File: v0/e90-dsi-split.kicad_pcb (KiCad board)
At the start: 2 copper layers, 33.9 x 22.1 mm, 12 parts, among them J1 3-2328724-1, J2 BM23PF0.8-40DP-0.35V_51_, J3 I2C Pinstack, J4 GPIO Pinstack

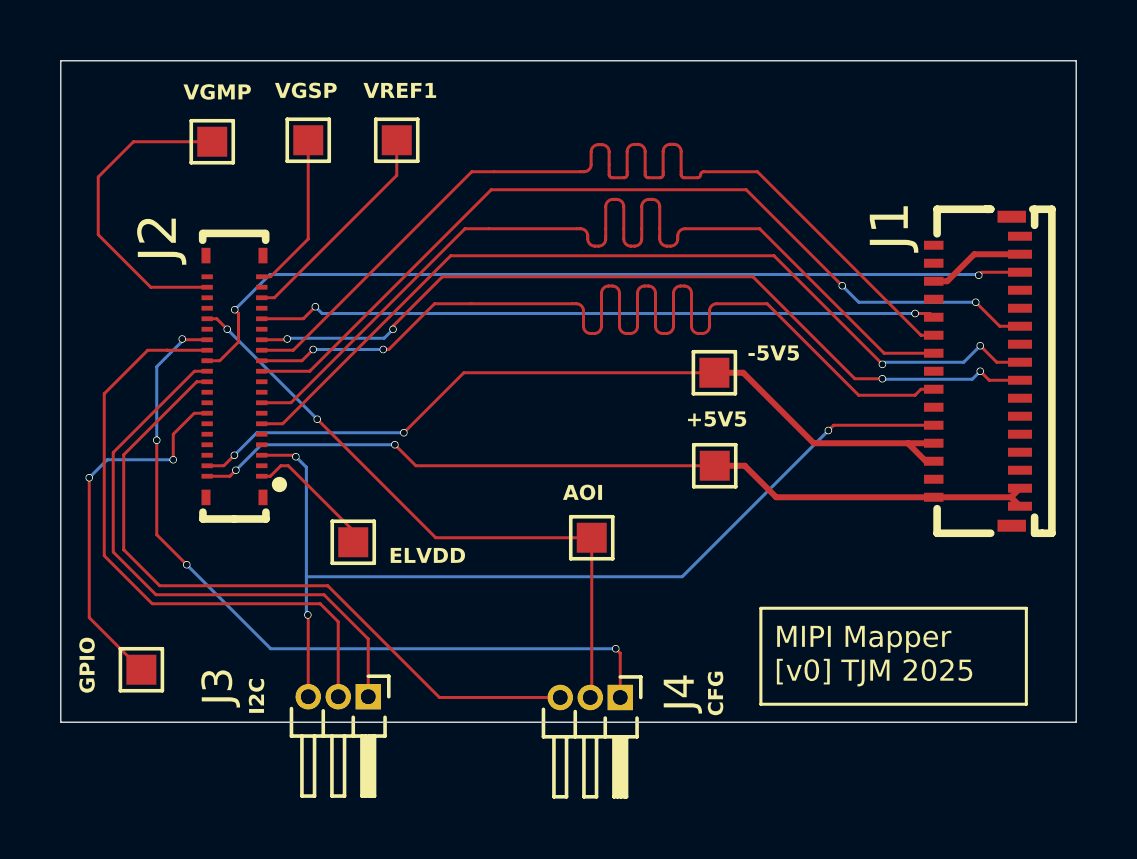
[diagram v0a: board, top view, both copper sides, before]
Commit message: next
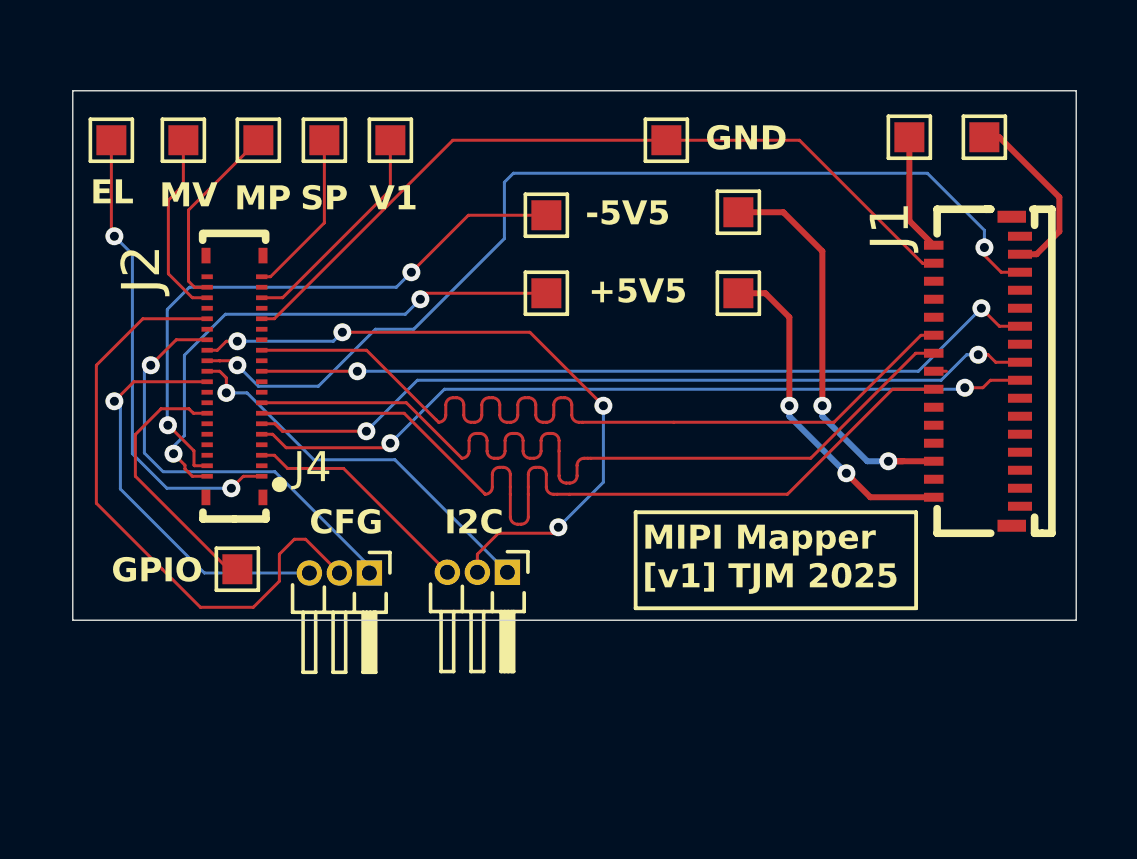
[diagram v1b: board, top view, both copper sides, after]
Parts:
- added TP10: +5V5 Src, TestPoint:TestPoint_Pad_1.0x1.0mm, F.Cu at (100.8, 54.2)
- added TP11: VDD3V3_SYS, TestPoint:TestPoint_Pad_1.0x1.0mm, F.Cu at (106.5, 49.0)
- added TP11: +5V5 Screen, TestPoint:TestPoint_Pad_1.0x1.0mm, F.Cu at (100.8, 51.5)
- added TP11: VDD3V3_SYS, TestPoint:TestPoint_Pad_1.0x1.0mm, F.Cu at (109.0, 49.0)
- added TP9: GND Test, TestPoint:TestPoint_Pad_1.0x1.0mm, F.Cu at (98.4, 49.1)
- TP1: value +5V5 Test -> +5V5 Screen
- TP2: value -5V5 Test -> -5V5 Screen
- TP3: value AOI Test -> MVDD Test
- moved TP3 19.0 mm to (82.3, 49.1)
- moved TP5 15.6 mm to (79.9, 49.1)
- moved J4 9.34 mm to (88.5, 63.5)
- moved TP1 8.04 mm to (94.4, 54.2)
- moved TP2 7.68 mm to (94.4, 51.6)
- moved J3 6.22 mm to (93.1, 63.5)
- moved TP6 4.63 mm to (84.1, 63.4)
- moved TP8 1.54 mm to (84.8, 49.1)
- moved TP7 0.54 mm to (87.0, 49.1)
- moved TP4 0.21 mm to (89.2, 49.1)
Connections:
- J1 pad 14: /DATAP2 -> /CLK_P
- J1 pad 15: /DATAN2 -> /CLK_N
- J2 pad 39: -5V5_BL -> /AVEE
- J2 pad 40: +5V5_BL -> /AVDD
- J2 pad 5: /CLKN -> /CLK_N
- J2 pad 7: /CLKP -> /CLK_P
- TP1 pad 1: +5V5_BL -> /AVDD
- TP2 pad 1: -5V5_BL -> /AVEE
- TP3 pad 1: /EN_AOI -> /MVDD
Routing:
- net /DATAP2: track 34.2 -> 0.00 mm, vias 2 -> 0
- net /CLK_P: track 0.00 -> 29.7 mm
- net /DATAN2: track 27.9 -> 0.00 mm, vias 4 -> 0
- net /CLK_N: track 0.00 -> 26.4 mm, vias 0 -> 2
- net GND: track 55.0 -> 34.8 mm, vias 5 -> 0
- net /AVEE: track 0.00 -> 20.0 mm, vias 0 -> 2
- net +5V5_BL: track 28.8 -> 10.9 mm
- net /AVDD: track 0.00 -> 17.9 mm, vias 0 -> 2
- net -5V5_BL: track 27.6 -> 13.3 mm
- net /IM_0: track 26.3 -> 14.5 mm, vias 4 -> 1
- net /ELVDD: track 4.48 -> 15.7 mm, vias 0 -> 2
- net /RL_SEL: track 23.5 -> 13.8 mm, vias 0 -> 1
- net /MVDD: track 0.00 -> 6.28 mm
- net /SCL: track 19.2 -> 13.1 mm, vias 0 -> 1
- net /VGMP: track 10.6 -> 6.37 mm
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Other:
- board size 33.9 x 22.1 mm -> 33.5 x 17.6 mm
- rule pad_to_mask_clearance: 0 -> 0.0508
- board text added: "EL"
- board text added: "GND"
- board text added: "MIPI Mapper [v1] TJM 2025"
- board text added: "MP"
- board text added: "MV"
- board text added: "SP"
- board text added: "V1"
- board text removed: "AOI"
- board text removed: "ELVDD"
- board text removed: "MIPI Mapper [v0] TJM 2025"
- board text removed: "VGMP"
- board text removed: "VGSP"
- board text removed: "VREF1"
